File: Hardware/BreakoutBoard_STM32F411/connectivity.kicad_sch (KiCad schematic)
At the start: 9 parts, among them J201 GSB1C41110SSHR, J202 PortB1, J203 PortB2, J204 PortA1, J205 PortA2, J206 SPI2, J207 PortA1

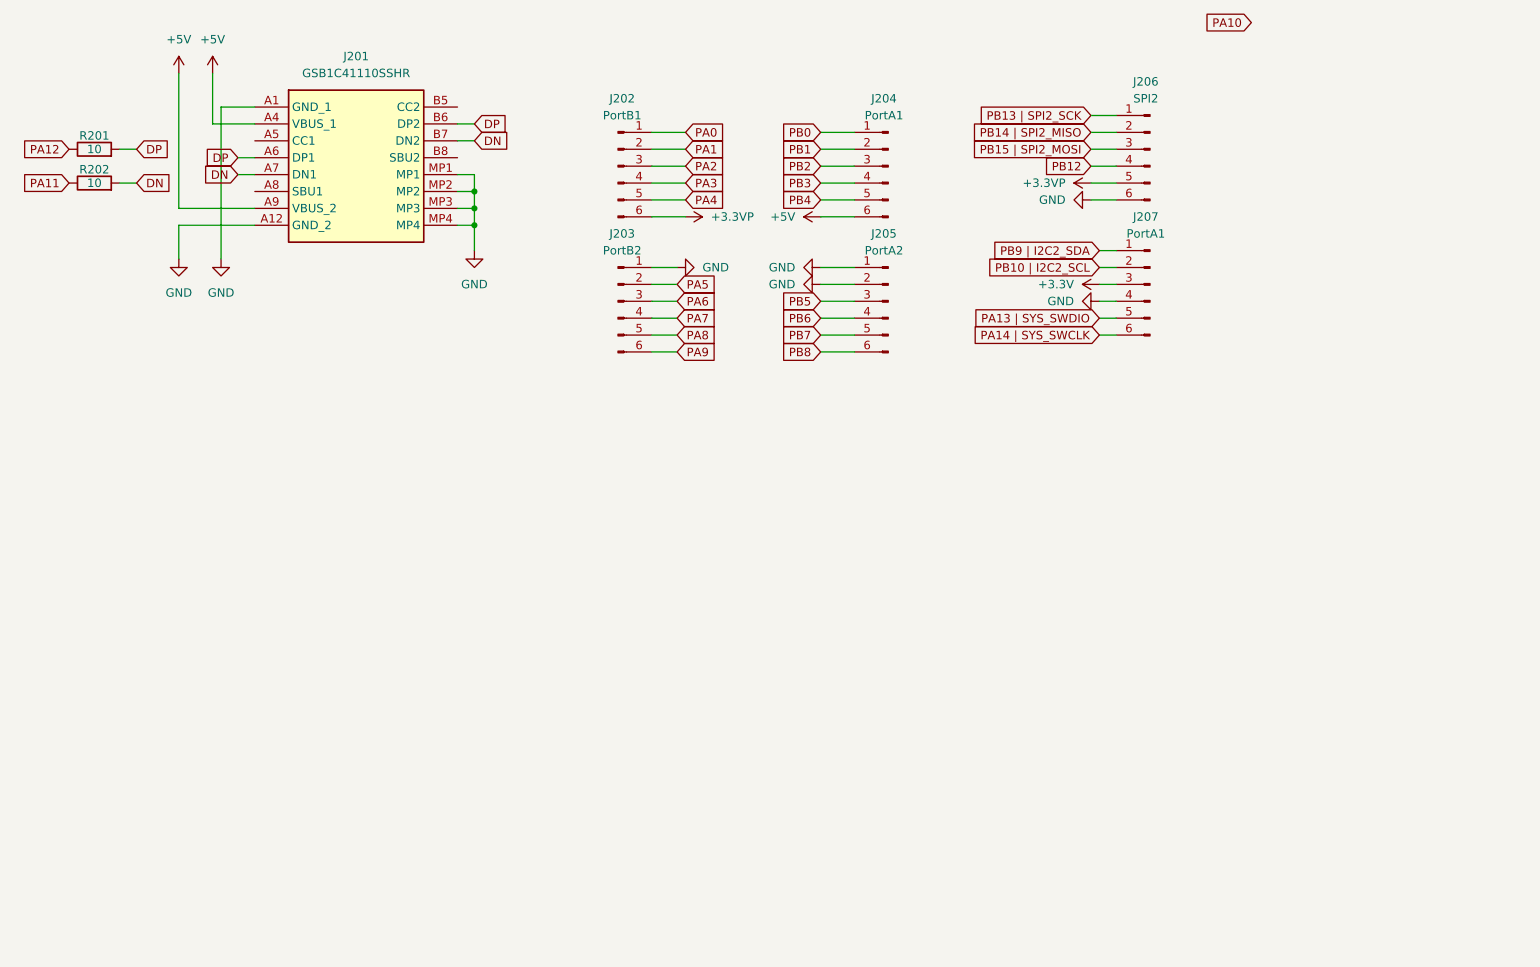
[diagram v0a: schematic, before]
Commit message: arranged:components (#3)
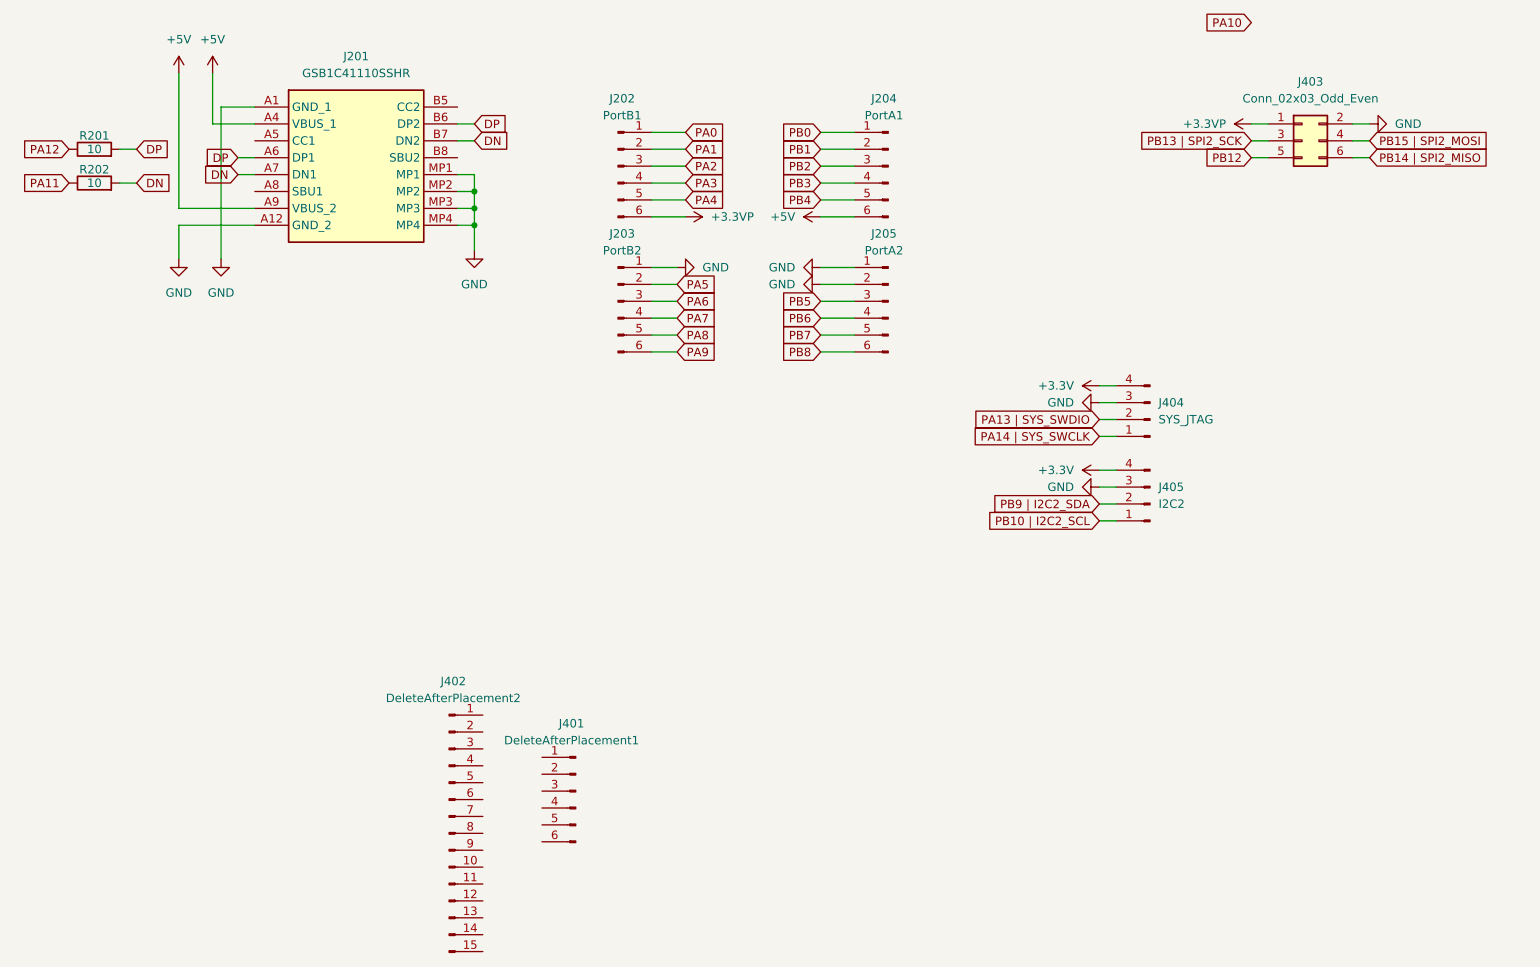
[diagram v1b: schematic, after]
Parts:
- removed J206: SPI2, Connector_PinHeader_2.54mm:PinHeader_1x06_P2.54mm_Vertical, symbol Connector:Conn_01x06_Pin
- removed J207: PortA1, Connector_PinHeader_2.54mm:PinHeader_1x06_P2.54mm_Vertical, symbol Connector:Conn_01x06_Pin
- added J401: DeleteAfterPlacement1, Connector_PinHeader_2.54mm:PinHeader_1x06_P2.54mm_Vertical, symbol Connector:Conn_01x06_Pin
- added J402: DeleteAfterPlacement2, Connector_PinHeader_2.54mm:PinHeader_1x15_P2.54mm_Vertical, symbol Connector:Conn_01x15_Pin
- added J403: Conn_02x03_Odd_Even, Connector_PinHeader_2.54mm:PinHeader_2x03_P2.54mm_Vertical, symbol Connector_Generic:Conn_02x03_Odd_Even
- added J404: SYS_JTAG, Connector_PinHeader_2.54mm:PinHeader_1x04_P2.54mm_Vertical, symbol Connector:Conn_01x04_Pin
- added J405: I2C2, Connector_PinHeader_2.54mm:PinHeader_1x04_P2.54mm_Vertical, symbol Connector:Conn_01x04_Pin
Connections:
- net +3.3V: now also J404.4 (Pin_4), J405.4 (Pin_4)
- net +3.3VP: now also J403.1 (Pin_1)
- net GND: now also J403.2 (Pin_2), J404.3 (Pin_3), J405.3 (Pin_3)
- net PA13 | SYS_SWDIO: now also J404.2 (Pin_2)
- net PA14 | SYS_SWCLK: now also J404.1 (Pin_1)
- net PB10 | I2C2_SCL: now also J405.1 (Pin_1)
- net PB12: now also J403.5 (Pin_5)
- net PB13 | SPI2_SCK: now also J403.3 (Pin_3)
- net PB14 | SPI2_MISO: now also J403.6 (Pin_6)
- net PB15 | SPI2_MOSI: now also J403.4 (Pin_4)
- net PB9 | I2C2_SDA: now also J405.2 (Pin_2)

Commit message: routed PCB (#4)
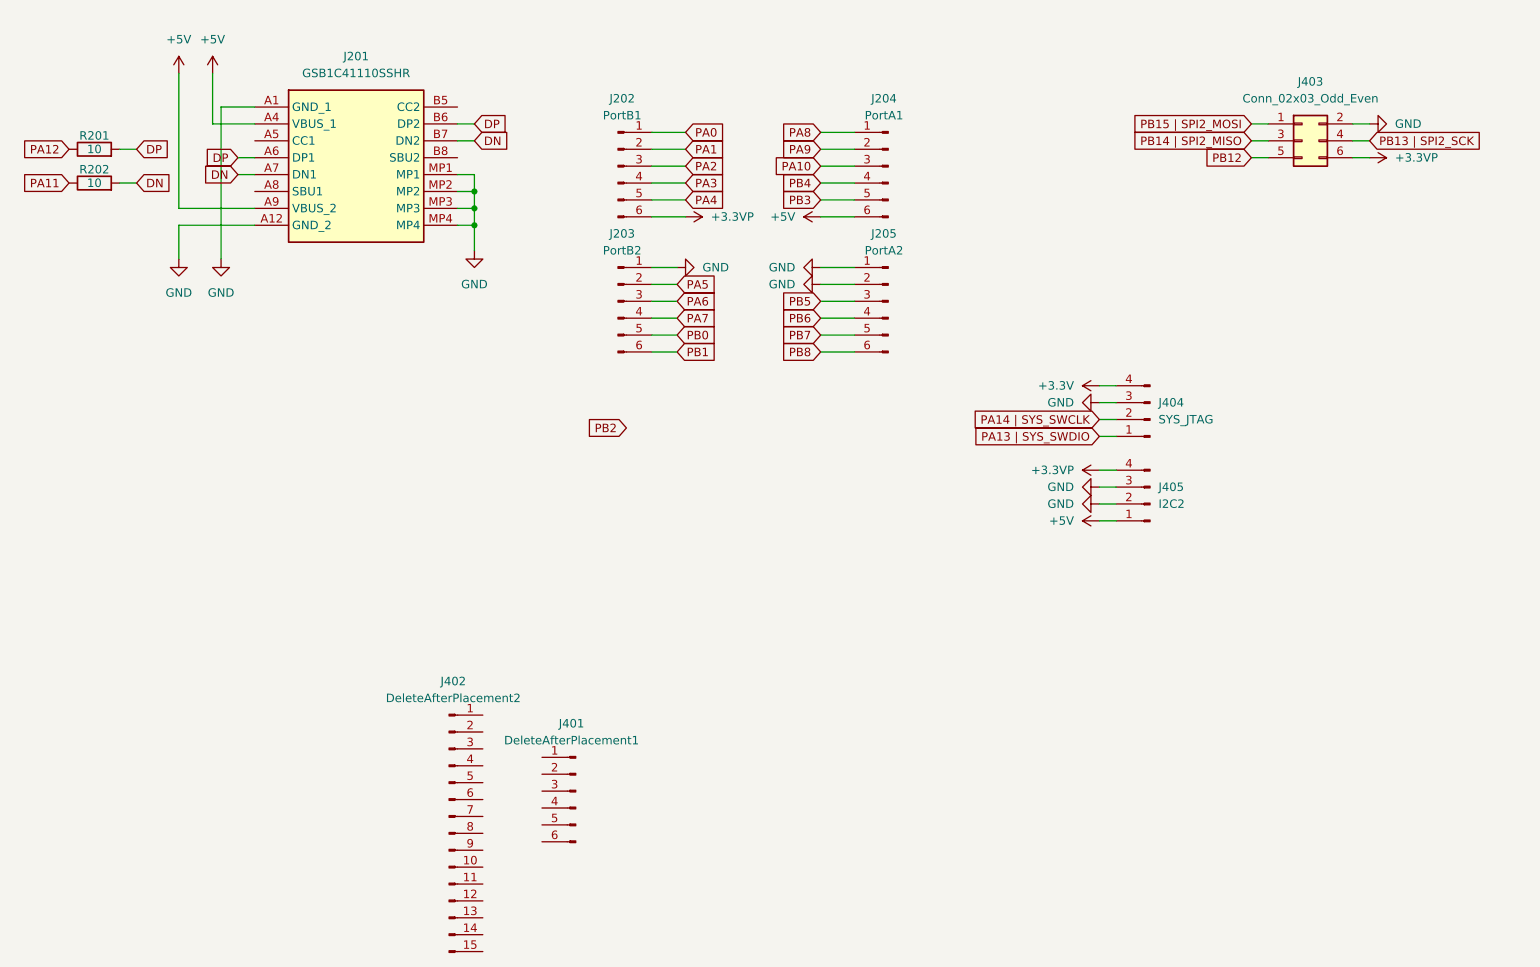
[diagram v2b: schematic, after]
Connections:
- net PB10 | I2C2_SCL is gone; now on net +5V: J405.1 (Pin_1)
- net PB9 | I2C2_SDA is gone; now on net GND: J405.2 (Pin_2)
- net +3.3V: no longer J405.4 (Pin_4)
- net +3.3VP: now also J403.6 (Pin_6), J405.4 (Pin_4); no longer J403.1 (Pin_1)
- net PA10: now also J204.3 (Pin_3)
- net PA13 | SYS_SWDIO: now also J404.1 (Pin_1); no longer J404.2 (Pin_2)
- net PA14 | SYS_SWCLK: now also J404.2 (Pin_2); no longer J404.1 (Pin_1)
- net PA8: now also J204.1 (Pin_1); no longer J203.5 (Pin_5)
- net PA9: now also J204.2 (Pin_2); no longer J203.6 (Pin_6)
- net PB0: now also J203.5 (Pin_5); no longer J204.1 (Pin_1)
- net PB1: now also J203.6 (Pin_6); no longer J204.2 (Pin_2)
- net PB13 | SPI2_SCK: now also J403.4 (Pin_4); no longer J403.3 (Pin_3)
- net PB14 | SPI2_MISO: now also J403.3 (Pin_3); no longer J403.6 (Pin_6)
- net PB15 | SPI2_MOSI: now also J403.1 (Pin_1); no longer J403.4 (Pin_4)
- net PB2: no longer J204.3 (Pin_3)
- net PB3: now also J204.5 (Pin_5); no longer J204.4 (Pin_4)
- net PB4: now also J204.4 (Pin_4); no longer J204.5 (Pin_5)
